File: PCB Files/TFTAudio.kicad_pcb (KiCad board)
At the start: 2 copper layers, 108 x 60.9 mm, 54 parts, among them J2 Lipo 1S, J3 Display, J4 AudioJack3, J5 expansion, J6 USB_C_Receptacle_USB2.0_14P, Q1 BSS138, Q2 BSS138, Q3 DMG2301L, SW1 SW_SPST, U1 ESP32-WROVER-E, U2 CH340C, U3 MCP73831-2-OT, U4 AP2112K-3.3, U5 PCM5102A

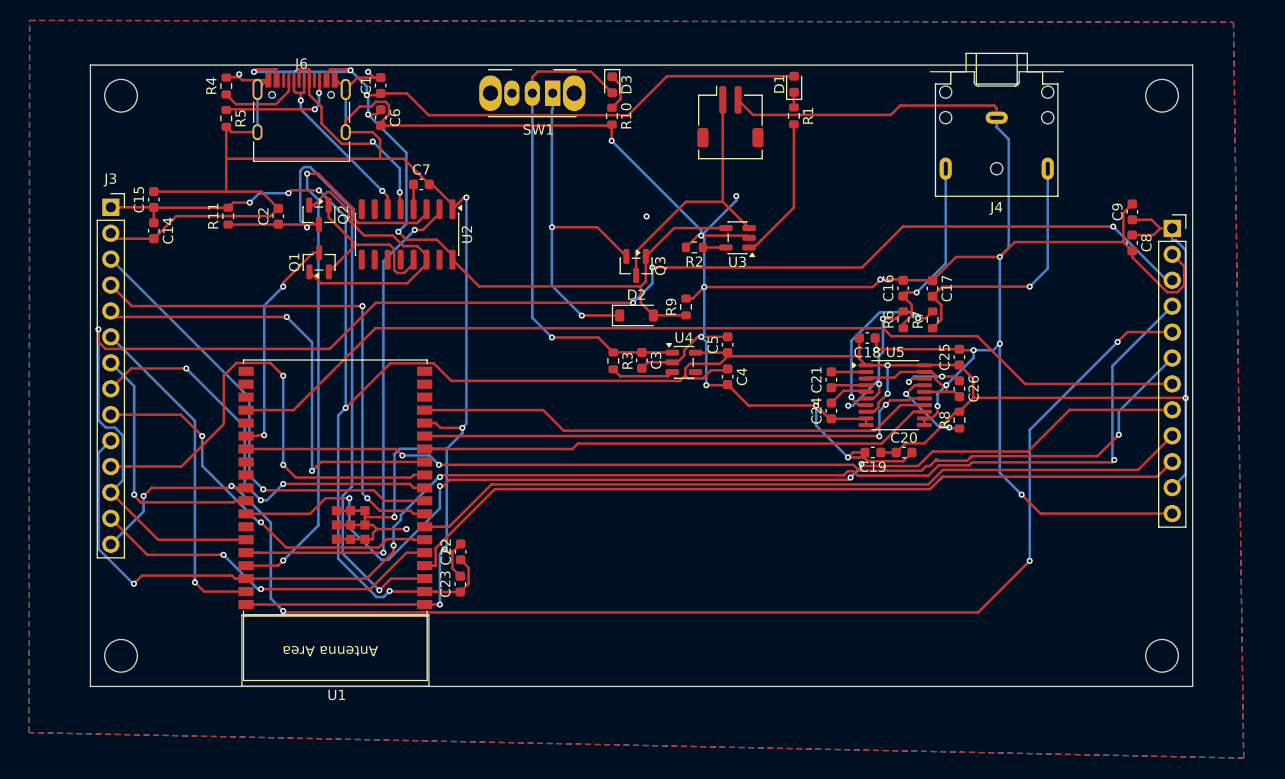
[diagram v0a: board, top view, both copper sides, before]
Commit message: PCB Draft 3
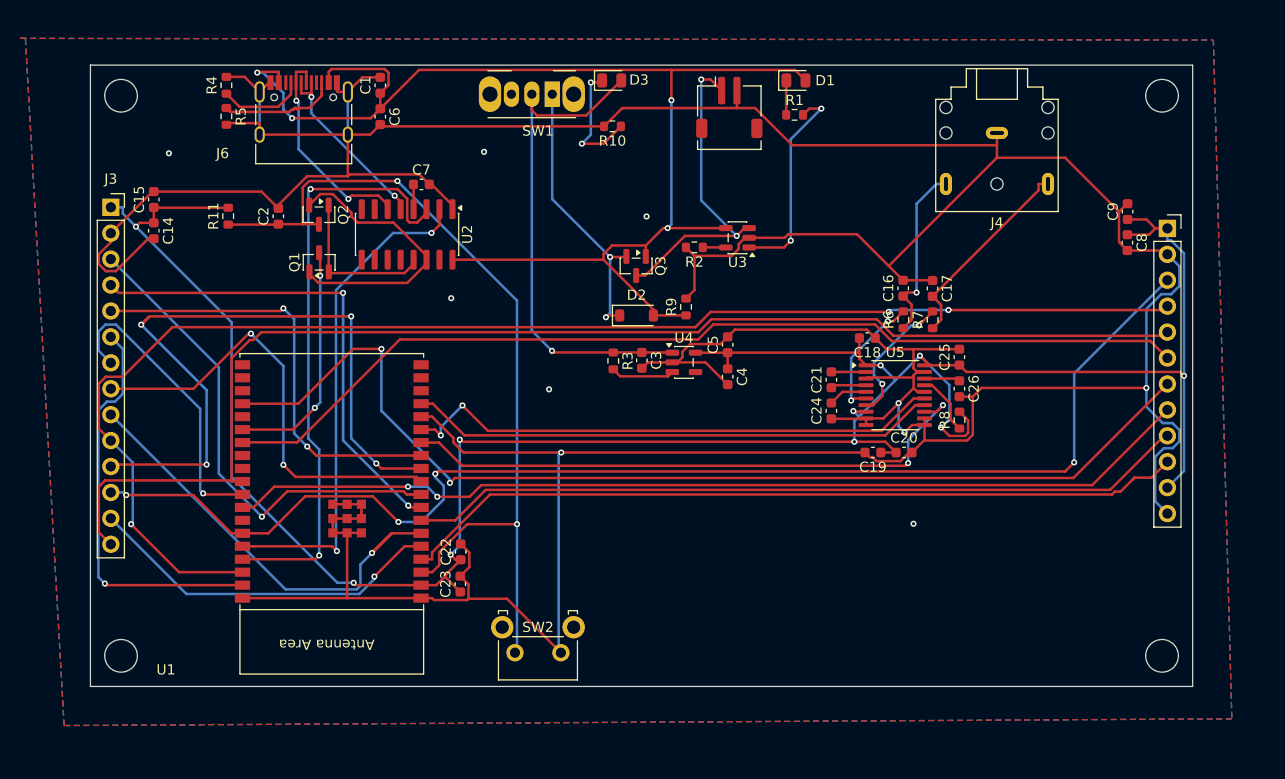
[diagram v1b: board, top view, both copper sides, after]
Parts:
- added SW2: RESET, Button_Switch_THT:SW_Tactile_SKHH_Angled, F.Cu at (59.1, 75.6)
- D1, D3: footprint LED_SMD:LED_0603_1608Metric -> LED_SMD:LED_0805_2012Metric
- U1: footprint Espressif:ESP32-WROVER-E -> PCM_Espressif:ESP32-WROVER-E
- moved J4 1.50 mm to (101.8, 24.6)
- moved R10 1.00 mm to (64.2, 24.0), turned to 180 degrees
- moved J2 0.92 mm to (75.6, 22.1)
- moved U1 0.72 mm to (36.6, 62.0)
- moved J5 0.47 mm to (118.5, 34.0)
- moved C9 0.47 mm to (114.6, 32.4)
- moved C8 0.47 mm to (114.6, 35.4)
- moved D3 0.43 mm to (64.1, 19.5), turned to 0 degrees
- moved D1 0.41 mm to (82.1, 19.5), turned to 0 degrees
- moved J6 0.32 mm to (33.9, 23.8)
- moved R5 0.20 mm to (26.3, 23.0)
- moved R1 0.13 mm to (82.0, 22.9), turned to 0 degrees
- moved C6 0.11 mm to (41.4, 23.1)
- moved SW1 0.11 mm to (58.2, 20.9)
- moved R4 0.08 mm to (26.3, 20.0)
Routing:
- net /CTP_SDA: track 147.9 -> 125.3 mm
- net /CTP_RST: track 47.6 -> 69.2 mm, vias 2 -> 4
- net /EN: track 66.4 -> 85.3 mm
- net +3.3V: track 228.0 -> 244.4 mm, vias 8 -> 10
- net /SD_CS: track 137.4 -> 126.6 mm, vias 5 -> 0
- net /GPIO15: track 96.3 -> 106.2 mm, vias 0 -> 2
- net Net-(D3-K): track 3.72 -> 12.1 mm, vias 0 -> 2
- net /MISO: track 38.2 -> 46.4 mm, vias 2 -> 1
- net /MOSI: track 32.9 -> 40.8 mm
- net /GPIO19: track 103.3 -> 95.4 mm, vias 4 -> 2
- net /SWIN: track 35.2 -> 27.4 mm
- net /BCK: track 50.5 -> 57.9 mm, vias 0 -> 2
- net Net-(U3-STAT): track 14.2 -> 20.6 mm, vias 0 -> 2
- net Net-(C17-Pad2): track 26.0 -> 20.1 mm, vias 1 -> 0
- net Net-(J2-Pin_1): track 26.5 -> 32.2 mm, vias 0 -> 2
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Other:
- outline, holes or cut-outs redrawn

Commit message: PCB draft 4
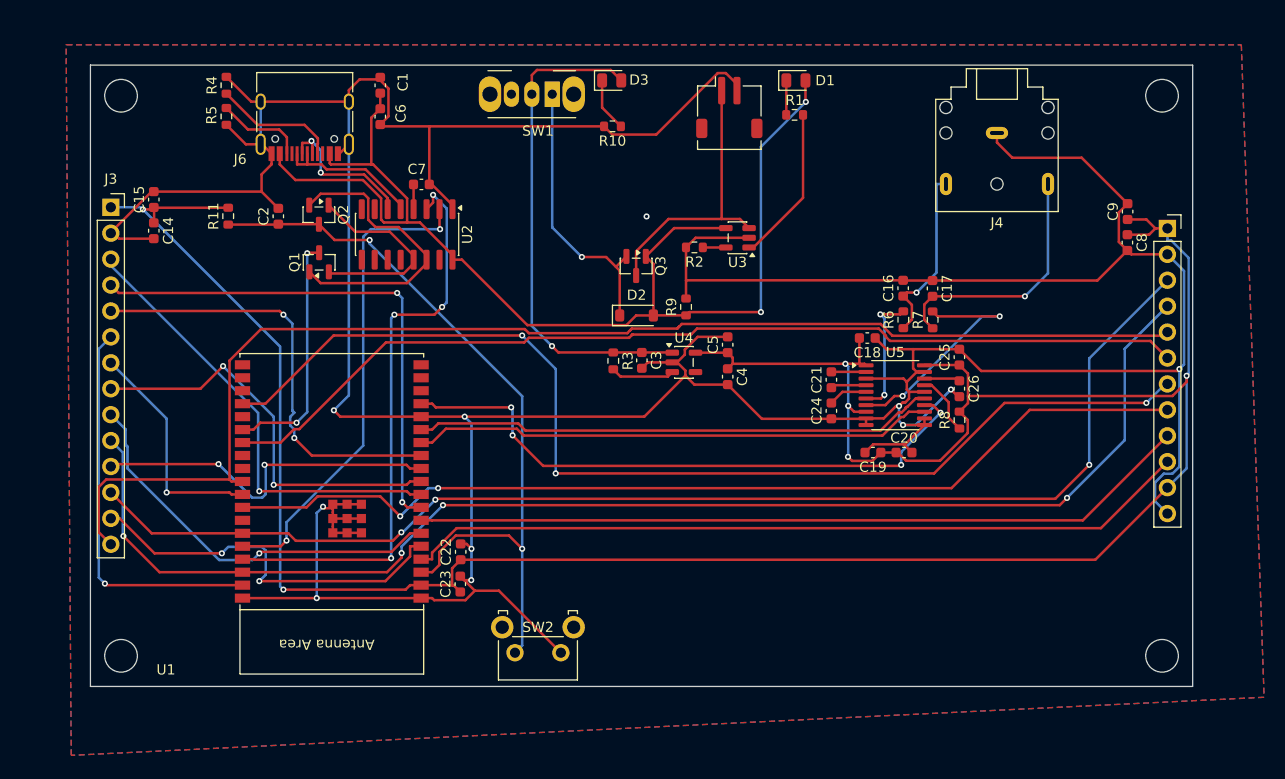
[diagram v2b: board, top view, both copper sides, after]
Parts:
- moved J6 1.13 mm to (34.0, 22.6), turned to 180 degrees
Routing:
- net /CTP_RST: track 69.2 -> 35.2 mm, vias 4 -> 2
- net GND: track 484.6 -> 463.2 mm, vias 4 -> 10
- net +3.3V: track 244.4 -> 263.0 mm, vias 10 -> 6
- net +5V: track 128.9 -> 116.0 mm, vias 4 -> 2
- net /EN: track 85.3 -> 74.1 mm
- net Net-(U5-OUTR): track 13.4 -> 23.5 mm
- net /DATA: track 51.8 -> 59.7 mm, vias 0 -> 4
- net /SCK: track 30.1 -> 22.5 mm
- net Net-(D3-K): track 12.1 -> 5.26 mm, vias 2 -> 0
- net /BCK: track 57.9 -> 51.1 mm, vias 2 -> 0
- net /MISO: track 46.4 -> 39.8 mm
- net Net-(U2-UD-): track 21.4 -> 15.5 mm
- net /CTP_SCL: track 135.9 -> 130.3 mm, vias 3 -> 4
- net Net-(U3-STAT): track 20.6 -> 15.4 mm, vias 2 -> 0
- net Net-(C17-Pad2): track 20.1 -> 24.8 mm, vias 0 -> 1
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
